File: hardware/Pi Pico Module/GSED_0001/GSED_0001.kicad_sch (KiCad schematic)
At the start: 17 parts, among them J1 Conn_01x10_Socket, J10 Ignition E-Match, J11 QD E-Match, J12 Radio, J14 Power Input, J2 Conn_01x10_Socket, J3 Conn_01x10_Socket (Digital), J4 K-Bottle PT, J5 Load Cell + Amp, J6 Tank PT, J7 Current Sensor, J8 K-Bottle TC, J9 Fill Servo, U1 BA90BC0FP-E2

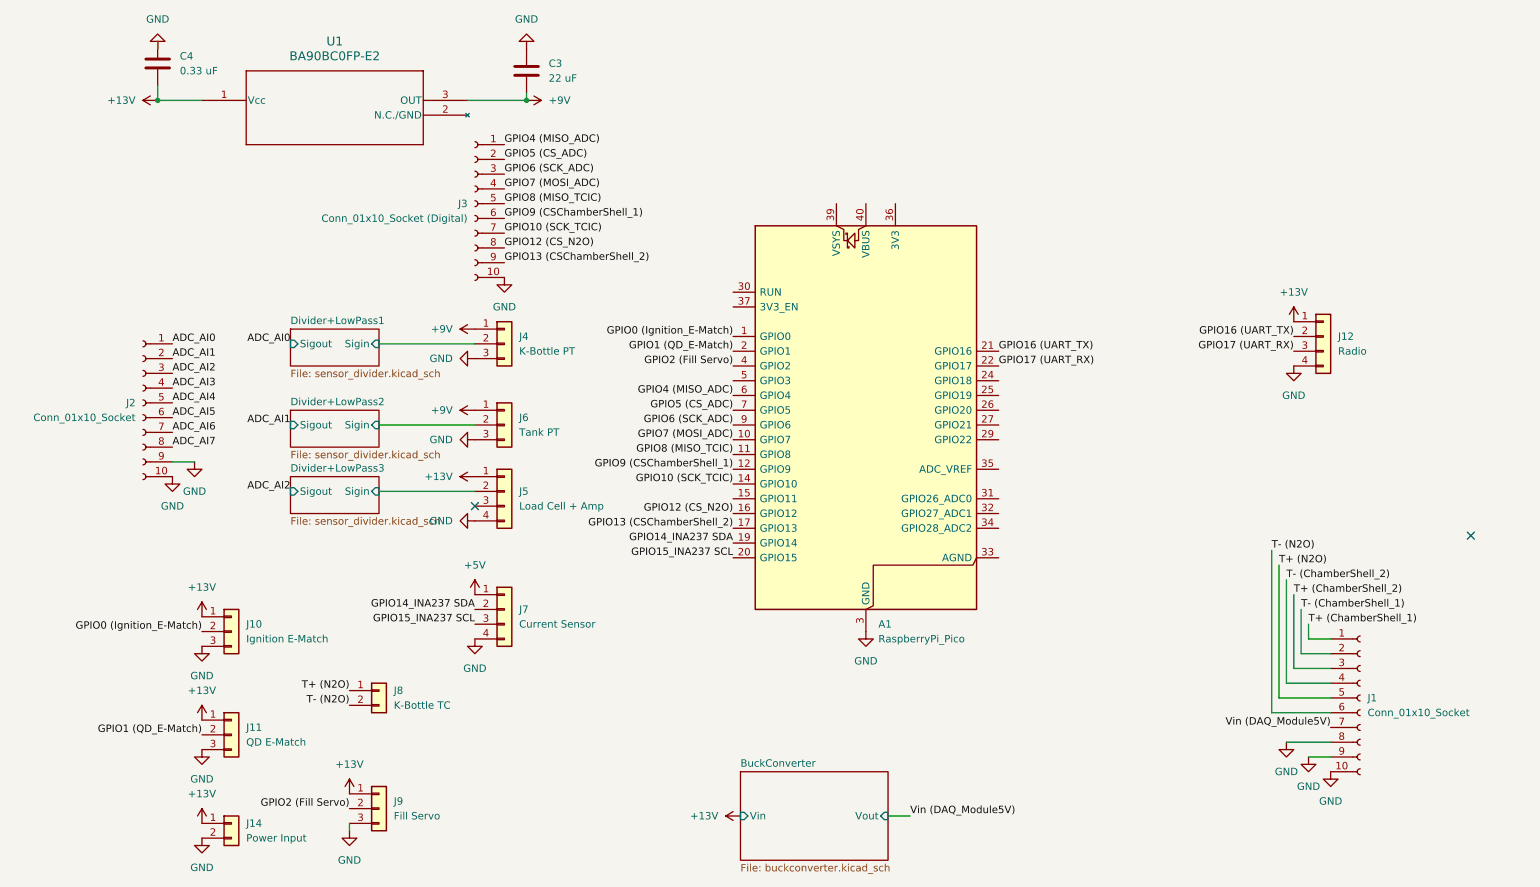
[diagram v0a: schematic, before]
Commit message: Reuploaded folder
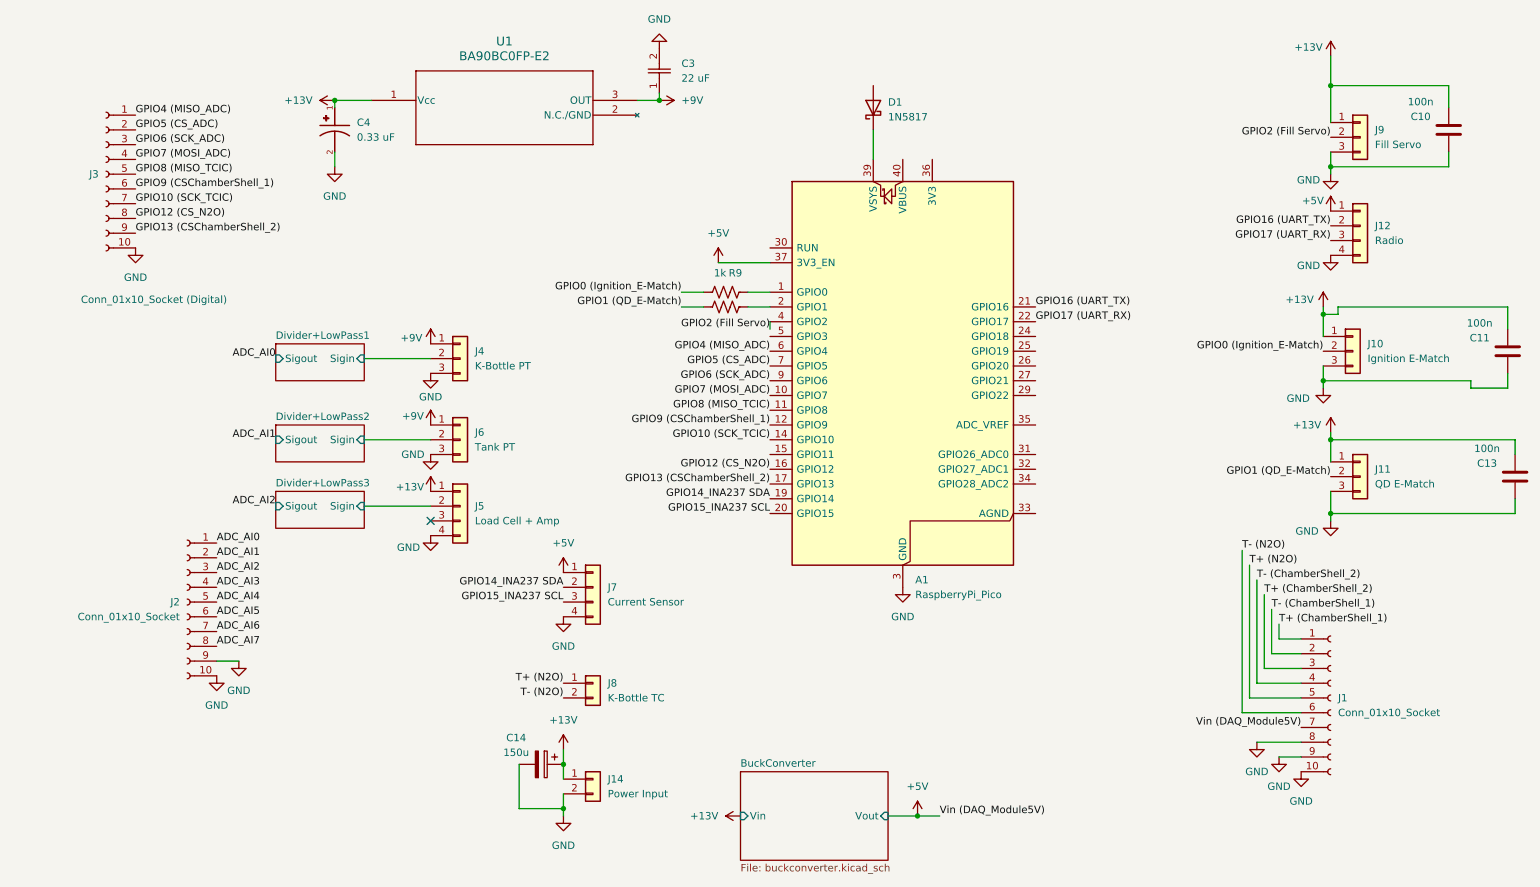
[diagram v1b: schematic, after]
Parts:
- added C10, C11, C13: 100n, Capacitor_SMD:C_0603_1608Metric, symbol Device:C
- added C14: 150u, EEUFC1H151B:CAPPRD500W60D1000H1600, symbol Device:C_Polarized
- added D1: 1N5817, Diode_THT:D_DO-41_SOD81_P10.16mm_Horizontal, symbol Diode:1N5817
- added R10, R9: 1k, Resistor_SMD:R_0603_1608Metric, symbol Device:R_US
- C3: footprint (none) -> Capacitor_SMD:C_0805_2012Metric; symbol Device:C -> 595D226X0050R2T:595D226X0050R2T
- C4: footprint (none) -> TAJA334K050RNJ:CAPMP3216X180N; symbol Device:C -> TAJA334K050RNJ:TAJA334K050RNJ; MANUFACTURER (none) -> AVX; MAXIMUM_PACKAGE_HEIGHT (none) -> 1.8 mm; PARTREV (none) -> 031320; STANDARD (none) -> IPC 7351B
- J1, J2, J3: footprint (none) -> Connector_PinHeader_2.54mm:PinHeader_1x10_P2.54mm_Vertical
- J10, J11, J4, J6, J9: footprint (none) -> Connector_PinHeader_2.54mm:PinHeader_1x03_P2.54mm_Vertical
- J12, J5, J7: footprint (none) -> Connector_PinHeader_2.54mm:PinHeader_1x04_P2.54mm_Vertical
- J14: footprint (none) -> Connector_AMASS:AMASS_XT30U-M_1x02_P5.0mm_Vertical
- J8: footprint (none) -> AM-K-PCB:AMKPCB
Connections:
- net Vin (DAQ_Module5V) is gone; now on net +5V: J1.7 (Pin_7)
- net +13V: now also C4.1, C10.2, C11.2, C13.2, C14.1; no longer C4.2, J12.1 (Pin_1)
- net +5V: now also A1.37 (3V3_EN), J12.1 (Pin_1)
- net +9V: now also C3.1; no longer C3.2
- net GND: now also C3.2, C4.2, C10.1, C11.1, C13.1, C14.2; no longer C3.1, C4.1
- net GPIO0 (Ignition_E-Match): now also R9.1; no longer A1.1 (GPIO0)
- net GPIO1 (QD_E-Match): now also R10.1; no longer A1.2 (GPIO1)
- net at A1.39 (VSYS): now also D1.1 (K)
- new net: A1.1 (GPIO0), R9.2
- new net: A1.2 (GPIO1), R10.2
- no-connect marks 2 -> 1
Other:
- company: (none) -> Rocket Design Team
- title: (none) -> Pi Pico Module
- moved on the sheet: A1, J1, J10, J11, J12, J14, J2, J3, J4, J5, J6, J7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
